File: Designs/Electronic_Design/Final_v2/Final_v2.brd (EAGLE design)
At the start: 145.3 x 65.8 mm, 5 parts

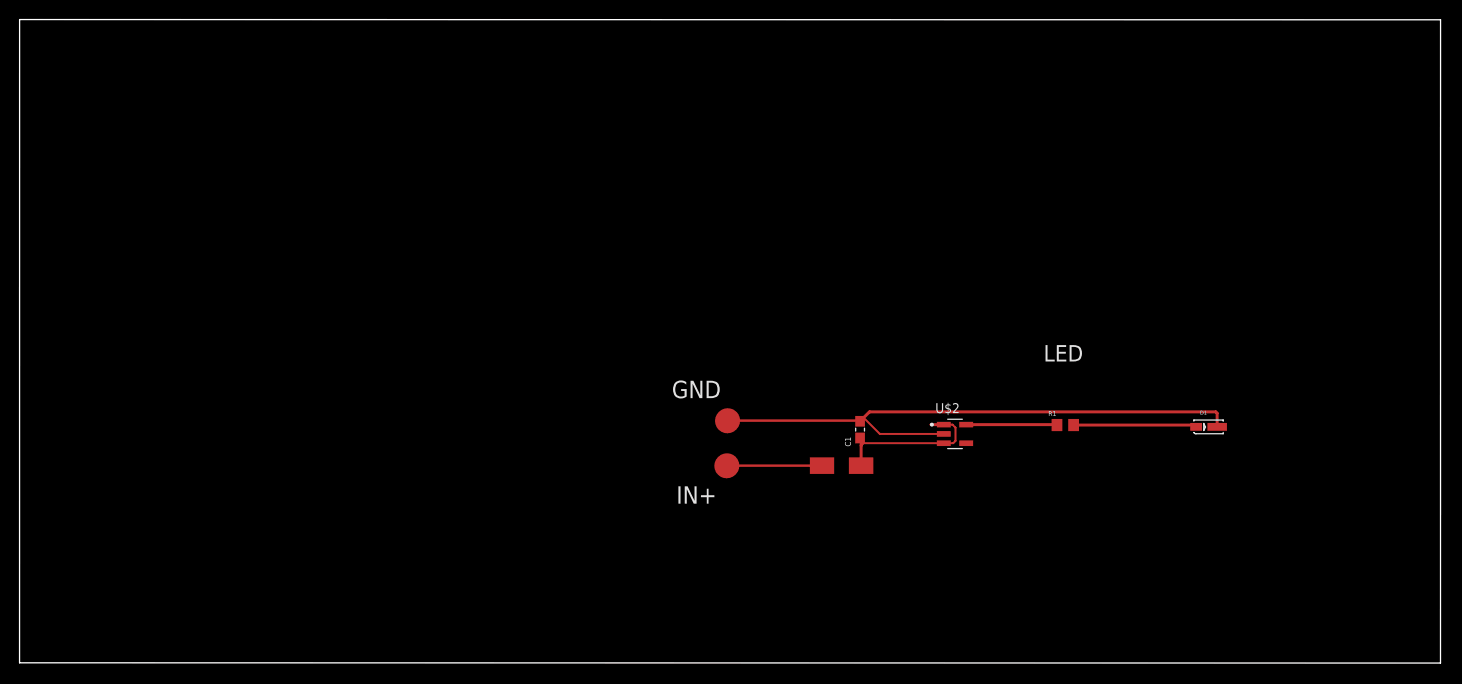
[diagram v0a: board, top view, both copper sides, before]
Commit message: Printings
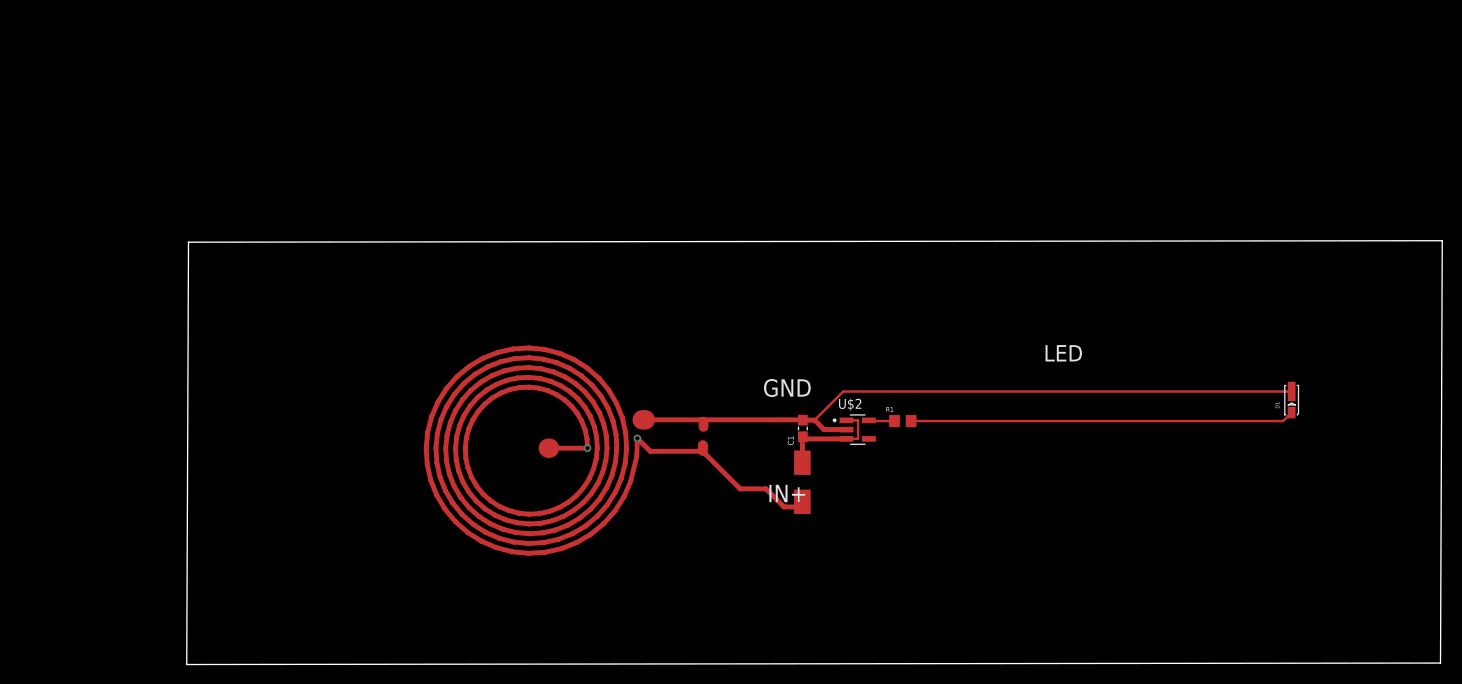
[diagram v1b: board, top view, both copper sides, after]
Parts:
- moved R1 16.6 mm to (74.3, 24.6)
- moved U$2 9.96 mm to (69.7, 23.8)
- moved D1 8.93 mm to (114.1, 26.8), turned to 90 degrees
- moved C1 5.85 mm to (64.1, 23.9)
- moved U$1 4.33 mm to (64.1, 18.4), turned to 90 degrees
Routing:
- net IN+: track 9.76 -> 292.5 mm, vias 0 -> 2
- net N$2: track 12.6 -> 39.3 mm
- net GND: track 61.3 -> 72.1 mm
- net N$1: track 9.30 -> 2.69 mm
- net N$4: track 16.7 -> 11.5 mm
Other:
- board size 145.3 x 65.8 mm -> 128.4 x 43.3 mm
